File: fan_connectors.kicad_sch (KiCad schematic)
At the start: 30 parts, among them Q1 CJ3134KW, Q2 AO3401A, Q3 CJ3134KW, Q4 AO3401A

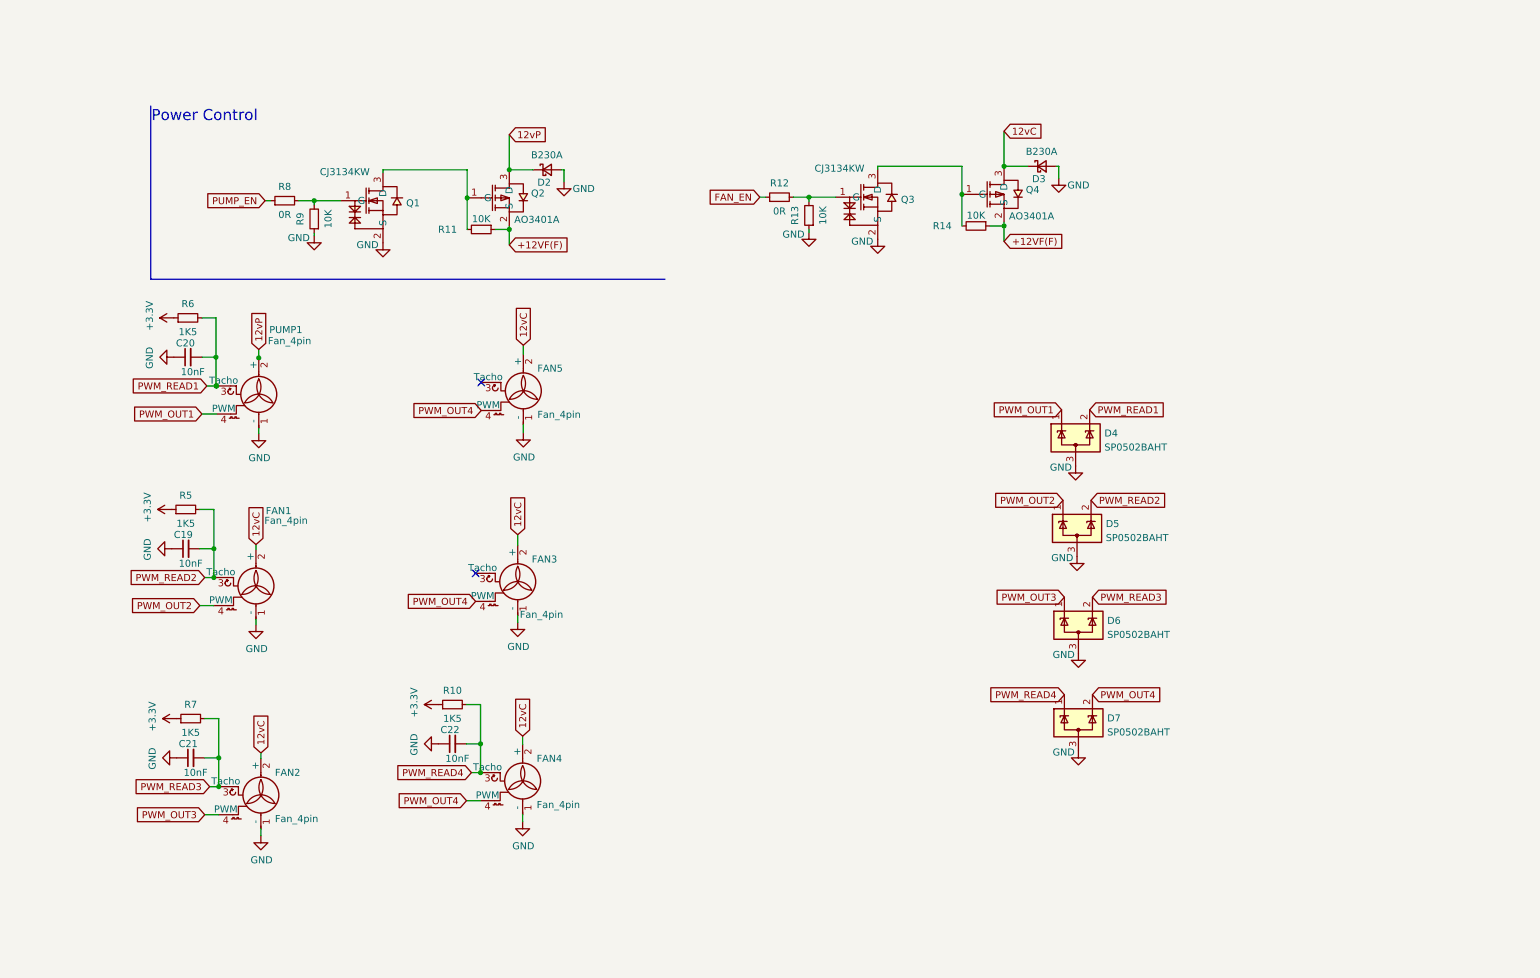
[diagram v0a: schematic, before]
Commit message: rev-7 ready
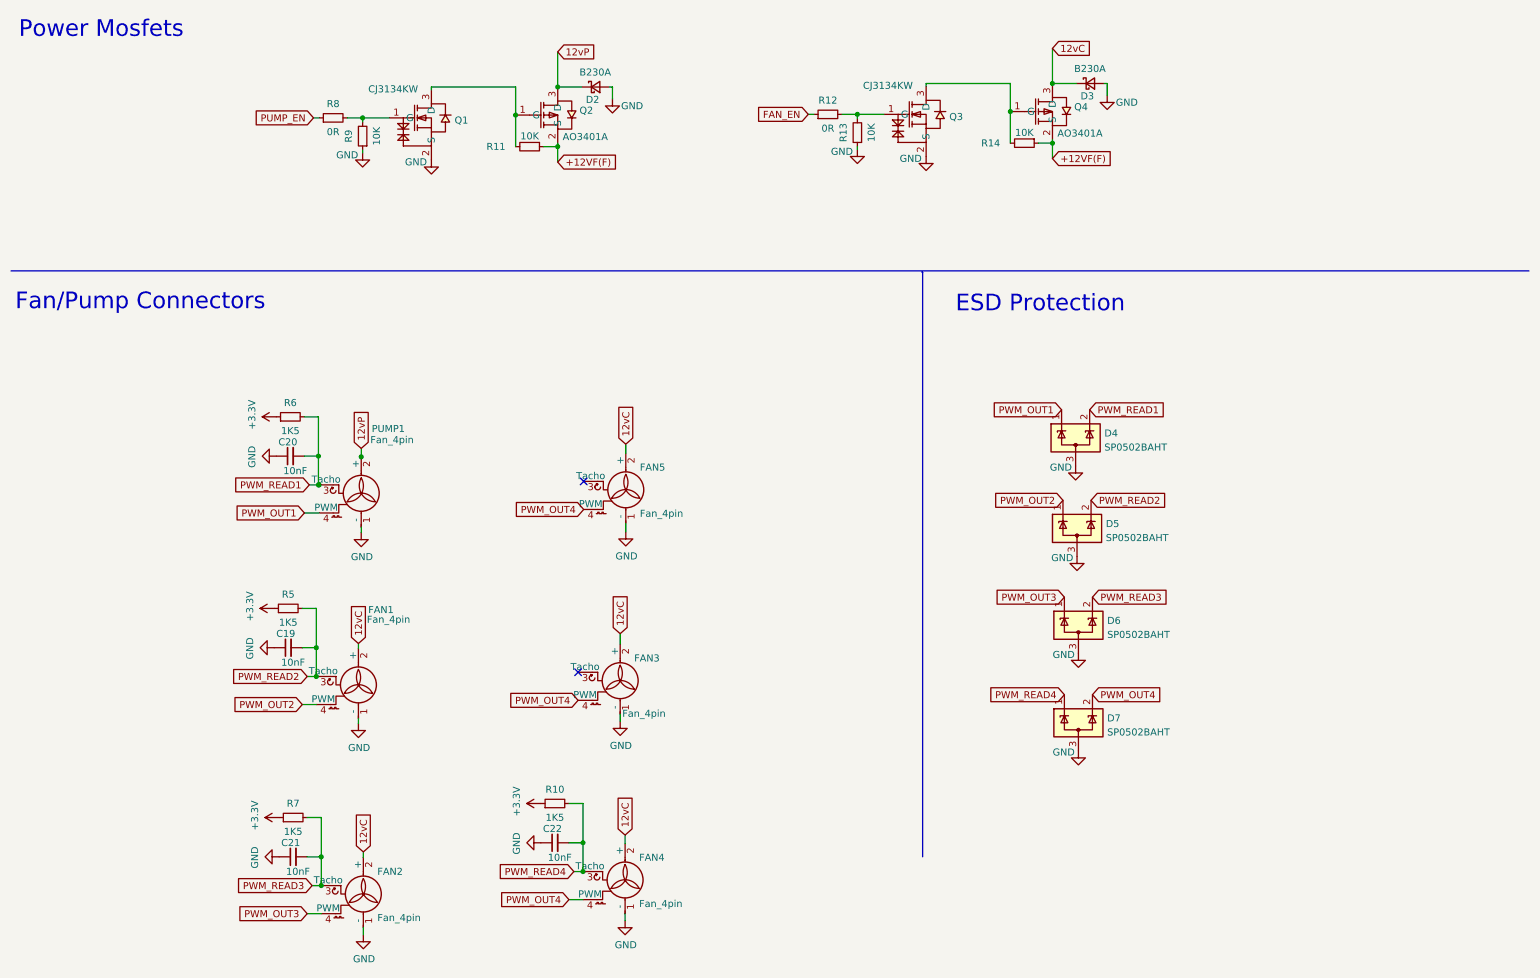
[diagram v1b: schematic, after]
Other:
- note added: "ESD Protection"
- note added: "Fan/Pump Connectors"
- note added: "Power Mosfets"
- note removed: "Power Control"
- moved on the sheet: C19, C20, C21, C22, D2, D3, FAN1, FAN2, FAN3, FAN4, FAN5, PUMP1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
